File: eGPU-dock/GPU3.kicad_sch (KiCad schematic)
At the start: 5 parts, among them U2 W25Q80DVSNIG

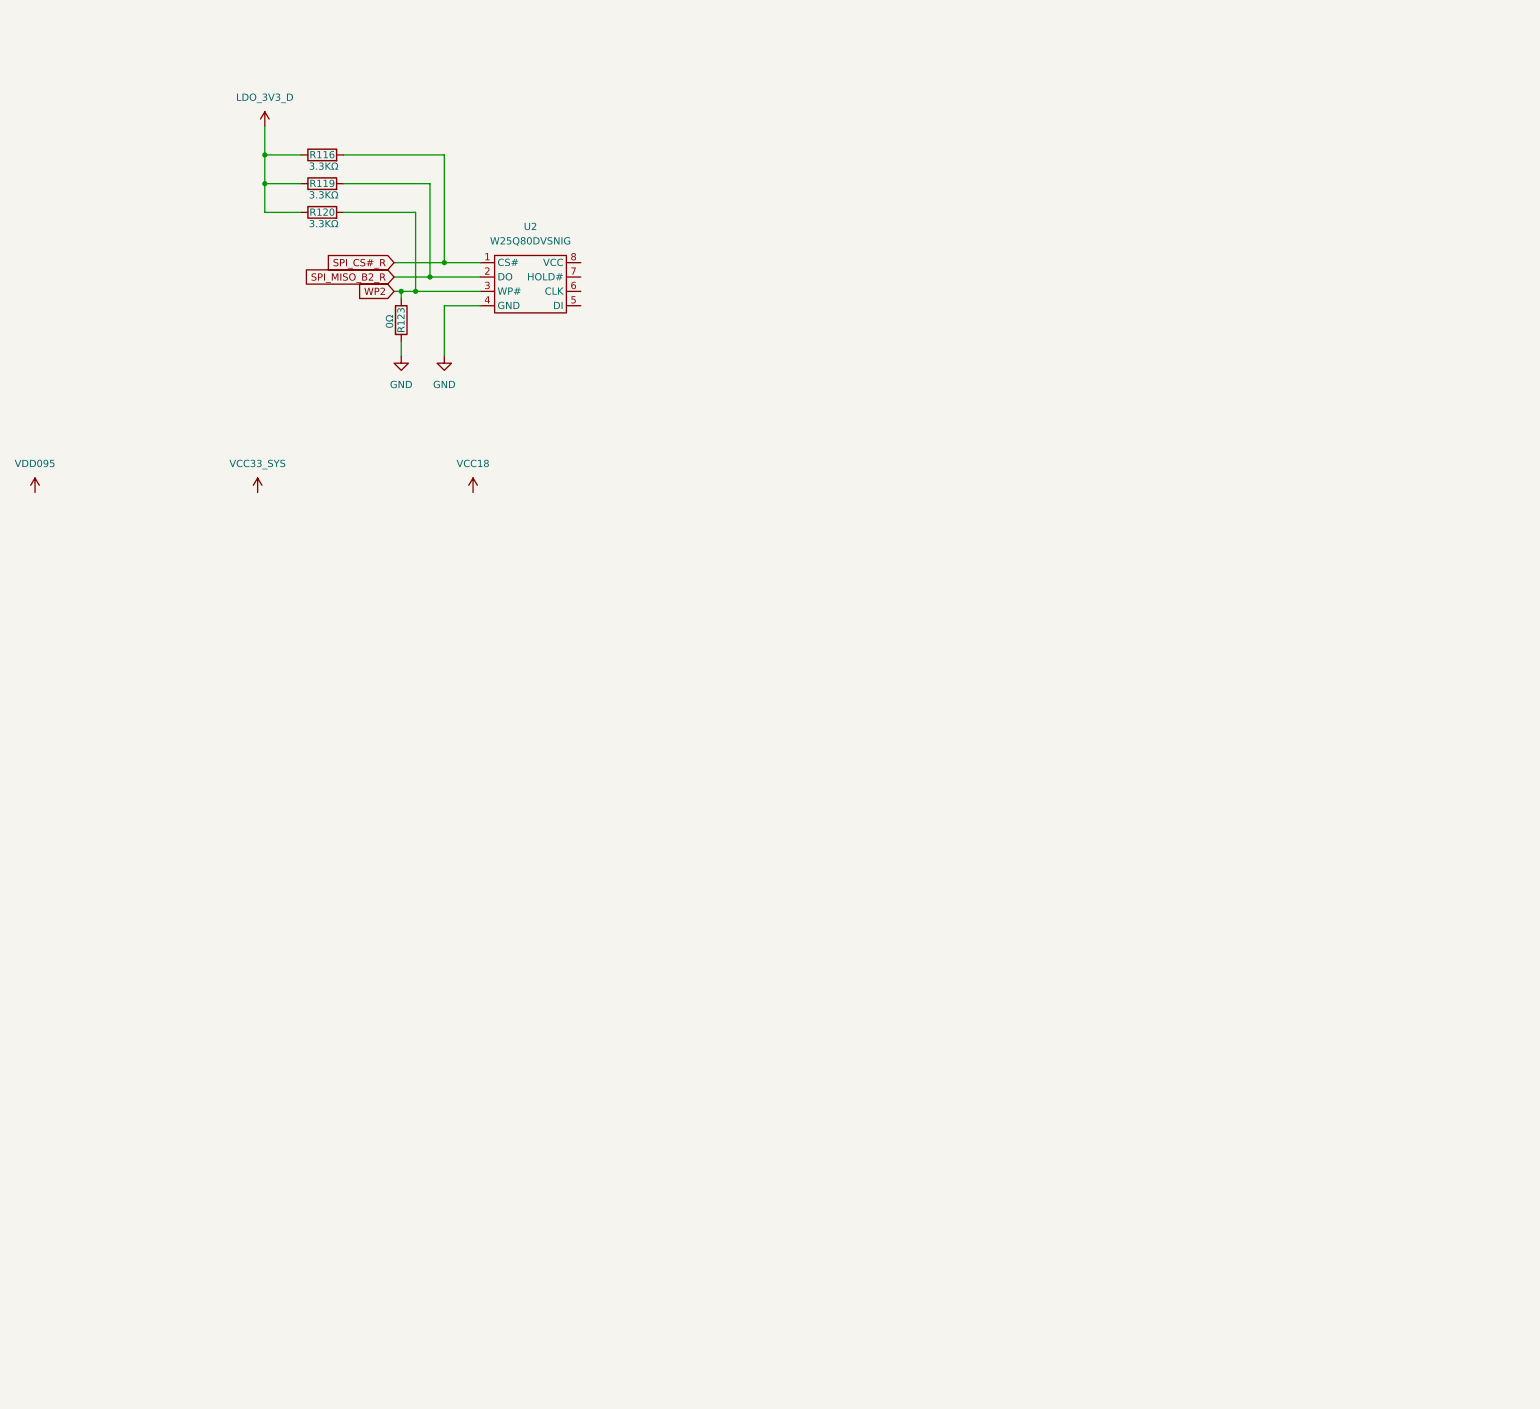
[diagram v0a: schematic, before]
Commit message: update
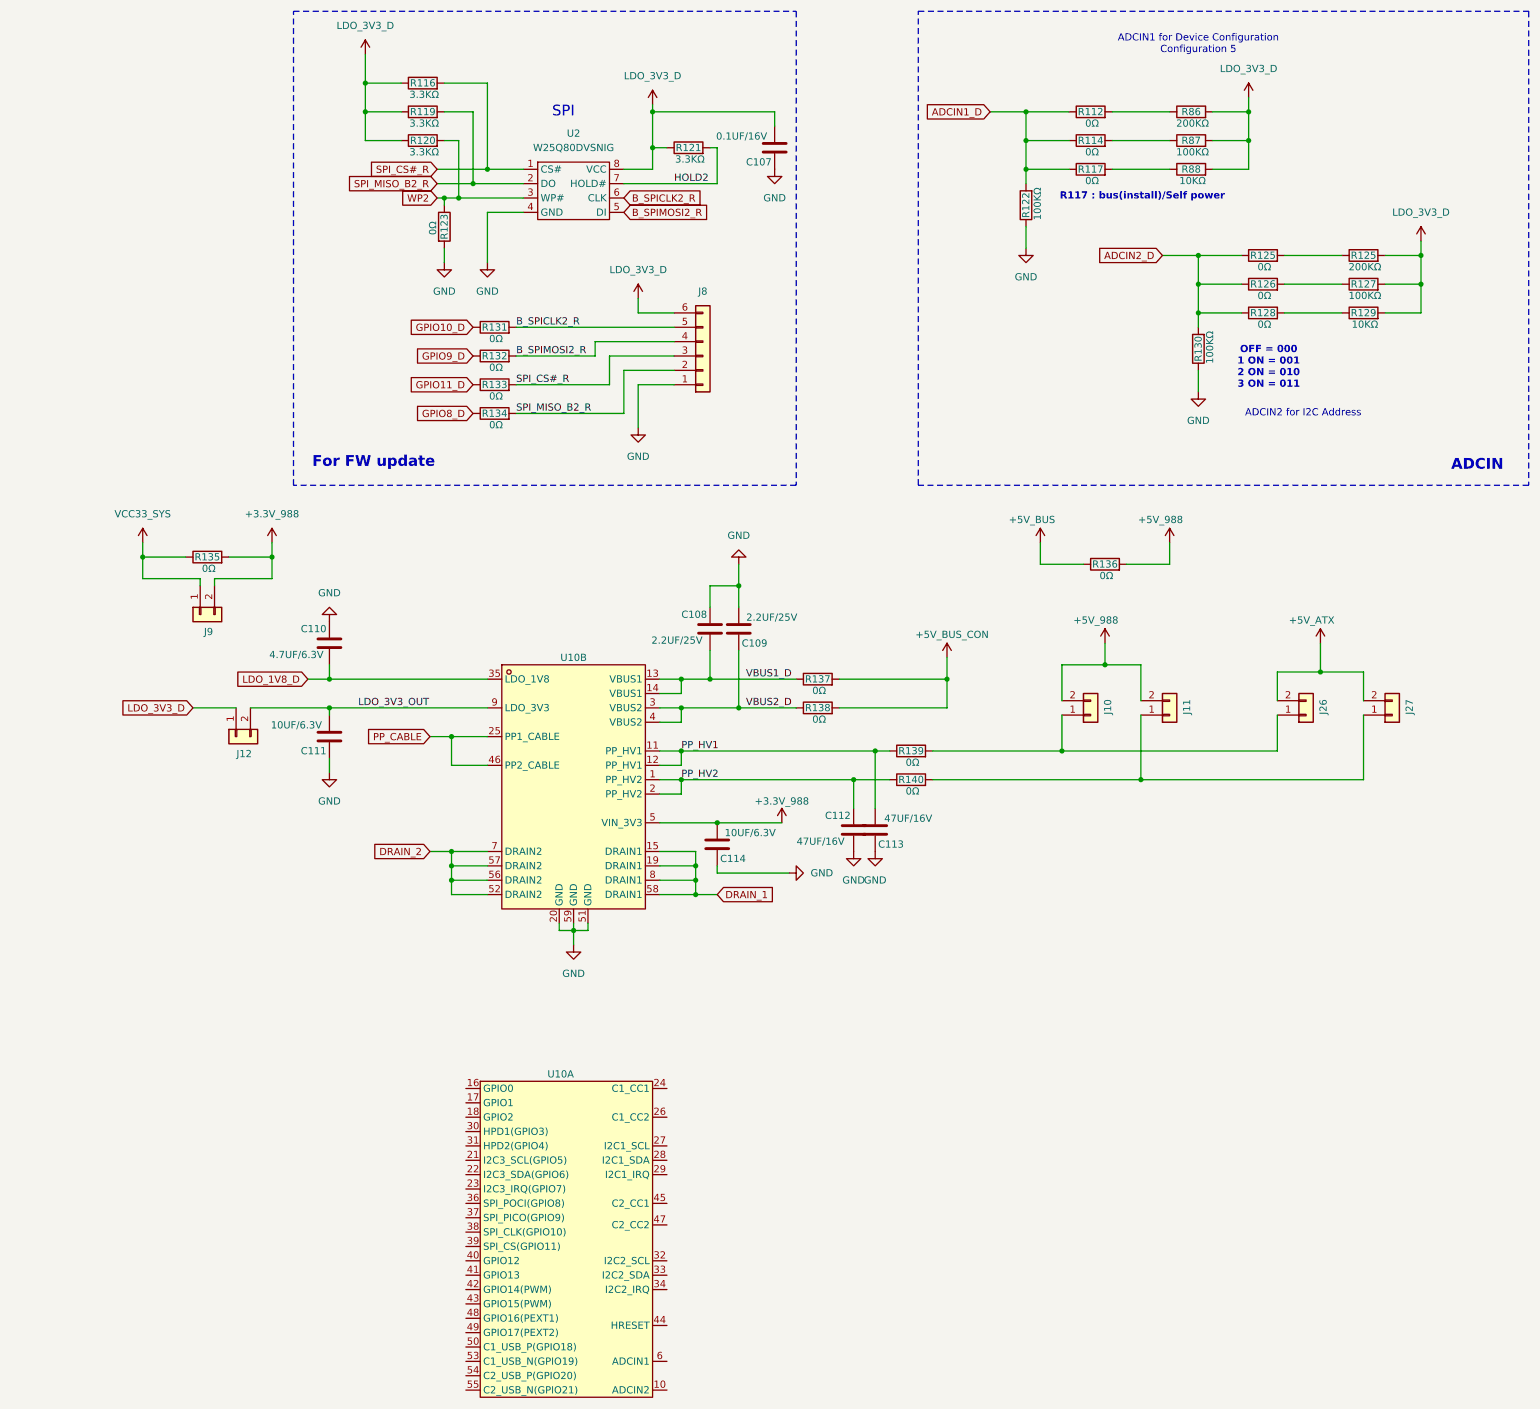
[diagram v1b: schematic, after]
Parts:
- added C107: 0.1UF/16V, Capacitor_SMD:C_0402_1005Metric, symbol Device:C
- added C108, C109: 2.2UF/25V, Capacitor_SMD:C_0402_1005Metric, symbol Device:C
- added C110: 4.7UF/6.3V, Capacitor_SMD:C_0402_1005Metric, symbol Device:C
- added C111, C114: 10UF/6.3V, Capacitor_SMD:C_0402_1005Metric, symbol Device:C
- added C112, C113: 47UF/16V, Capacitor_SMD:C_0402_1005Metric, symbol Device:C
- added J10, J11, J12, J26, J27, J9: Conn_01x02, Connector_PinHeader_2.54mm:PinHeader_1x02_P2.54mm_Vertical, symbol Connector_Generic:Conn_01x02
- added J8: Conn_01x06, symbol Connector_Generic:Conn_01x06
- added R112, R114, R117, R125, R126, R128, R131, R132, R133, R134, R135, R136, R137, R138, R139, R140: 0Ω, Resistor_SMD:R_0402_1005Metric, symbol Device:R
- added R121: 3.3KΩ, Resistor_SMD:R_0402_1005Metric, symbol Device:R
- added R122, R127, R130, R87: 100KΩ, Resistor_SMD:R_0402_1005Metric, symbol Device:R
- added R125, R86: 200KΩ, Resistor_SMD:R_0402_1005Metric, symbol Device:R
- added R129, R88: 10KΩ, Resistor_SMD:R_0402_1005Metric, symbol Device:R
- added U10: ~, eGPUlib:TPS65988DK, symbol egpulib:TPS65988DKRSHR
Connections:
- net GND: now also C107.1, C108.1, C109.2, C110.1, C111.1, C112.2, C113.1, C114.1, J8.1 (Pin_1), R122.1, R130.1, U10.20 (GND), U10.51 (GND), U10.59 (GND)
- net LDO_3V3_D: now also U2.8 (VCC), C107.2, J12.1 (Pin_1), J8.6 (Pin_6), R121.1, R125.2, R127.2, R129.2, R86.2, R87.2, R88.2
- net SPI_CS#_R: now also J8.3 (Pin_3), R133.2
- net SPI_MISO_B2_R: now also J8.2 (Pin_2), R134.2
- net VCC33_SYS: now also J9.1 (Pin_1), R135.1
- net B_SPIMOSI2_R: now reaches U2.5 (DI)
- net B_SPIMOSI2_R: now also J8.4 (Pin_4), R132.2
- net B_SPICLK2_R: now reaches U2.6 (CLK)
- net B_SPICLK2_R: now also J8.5 (Pin_5), R131.2
- net HOLD2: now reaches U2.7 (HOLD#)
- net HOLD2: now also R121.2
- new net: R112.2, R86.1
- new net: J10.1 (Pin_1), J26.1 (Pin_1), R139.2
- new net: R126.2, R127.1
- new net: R114.2, R87.1
- new net: R128.2, R129.1
- new net: R117.2, R88.1
- new net: J11.1 (Pin_1), J27.1 (Pin_1), R140.2
- new net: R125.1, R125.2
- new net +3.3V_988: C114.2, J9.2 (Pin_2), R135.2, U10.5 (VIN_3V3)
- new net +5V_988: J10.2 (Pin_2), J11.2 (Pin_2), R136.2
- new net +5V_ATX: J26.2 (Pin_2), J27.2 (Pin_2)
- new net +5V_BUS: R136.1
- new net +5V_BUS_CON: R137.2, R138.2
- new net ADCIN1_D: R112.1, R114.1, R117.1, R122.2
- new net ADCIN2_D: R125.1, R126.1, R128.1, R130.2
- new net DRAIN_1: U10.15 (DRAIN1), U10.19 (DRAIN1), U10.58 (DRAIN1), U10.8 (DRAIN1)
- new net DRAIN_2: U10.52 (DRAIN2), U10.56 (DRAIN2), U10.57 (DRAIN2), U10.7 (DRAIN2)
- new net GPIO10_D: R131.1
- new net GPIO11_D: R133.1
- new net GPIO8_D: R134.1
- new net GPIO9_D: R132.1
- new net LDO_1V8_D: C110.2, U10.35 (LDO_1V8)
- new net LDO_3V3_OUT: C111.2, J12.2 (Pin_2), U10.9 (LDO_3V3)
- new net PP_CABLE: U10.25 (PP1_CABLE), U10.46 (PP2_CABLE)
- new net PP_HV1: C113.2, R139.1, U10.11 (PP_HV1), U10.12 (PP_HV1)
- new net PP_HV2: C112.1, R140.1, U10.1 (PP_HV2), U10.2 (PP_HV2)
- new net VBUS1_D: C108.2, R137.1, U10.13 (VBUS1), U10.14 (VBUS1)
- new net VBUS2_D: C109.1, R138.1, U10.3 (VBUS2), U10.4 (VBUS2)
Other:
- note added: "ADCIN"
- note added: "ADCIN1 for Device Configuration Configuration 5"
- note added: "ADCIN2 for I2C Address"
- note added: "For FW update"
- note added: "OFF = 000 1 ON = 001 2 ON = 010 3 ON = 011"
- note added: "R117 : bus(install)/Self power"
- note added: "SPI"
- moved on the sheet: R116, R119, R120, R123, U2
